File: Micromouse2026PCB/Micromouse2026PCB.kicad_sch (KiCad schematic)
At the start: 15 parts, among them J1 Power Terminal, J2 i2c OLED, J3 BNO085, SW1 RotaryEncoder_Switch, U6 L7805

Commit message: PCB work
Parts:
- J2: footprint Connector_PinHeader_2.54mm:PinHeader_1x04_P2.54mm_Vertical -> CustomFootprints:OLED_0.96_SSD1306_I2C
- J3: footprint Connector_PinHeader_2.54mm:PinHeader_1x06_P2.54mm_Vertical -> CustomFootprints:Adafruit_BNO085
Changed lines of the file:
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@@
 			)
 		)
-		(property "Footprint" "Connector_PinHeader_2.54mm:PinHeader_1x06_P2.54mm_Vertical"
+		(property "Footprint" "CustomFootprints:Adafruit_BNO085"
 			(at 101.6 48.26 0)
 			(hide yes)
@@
 			)
 		)
-		(property "Footprint" "Connector_PinHeader_2.54mm:PinHeader_1x04_P2.54mm_Vertical"
+		(property "Footprint" "CustomFootprints:OLED_0.96_SSD1306_I2C"
 			(at 101.6 69.85 0)
 			(hide yes)

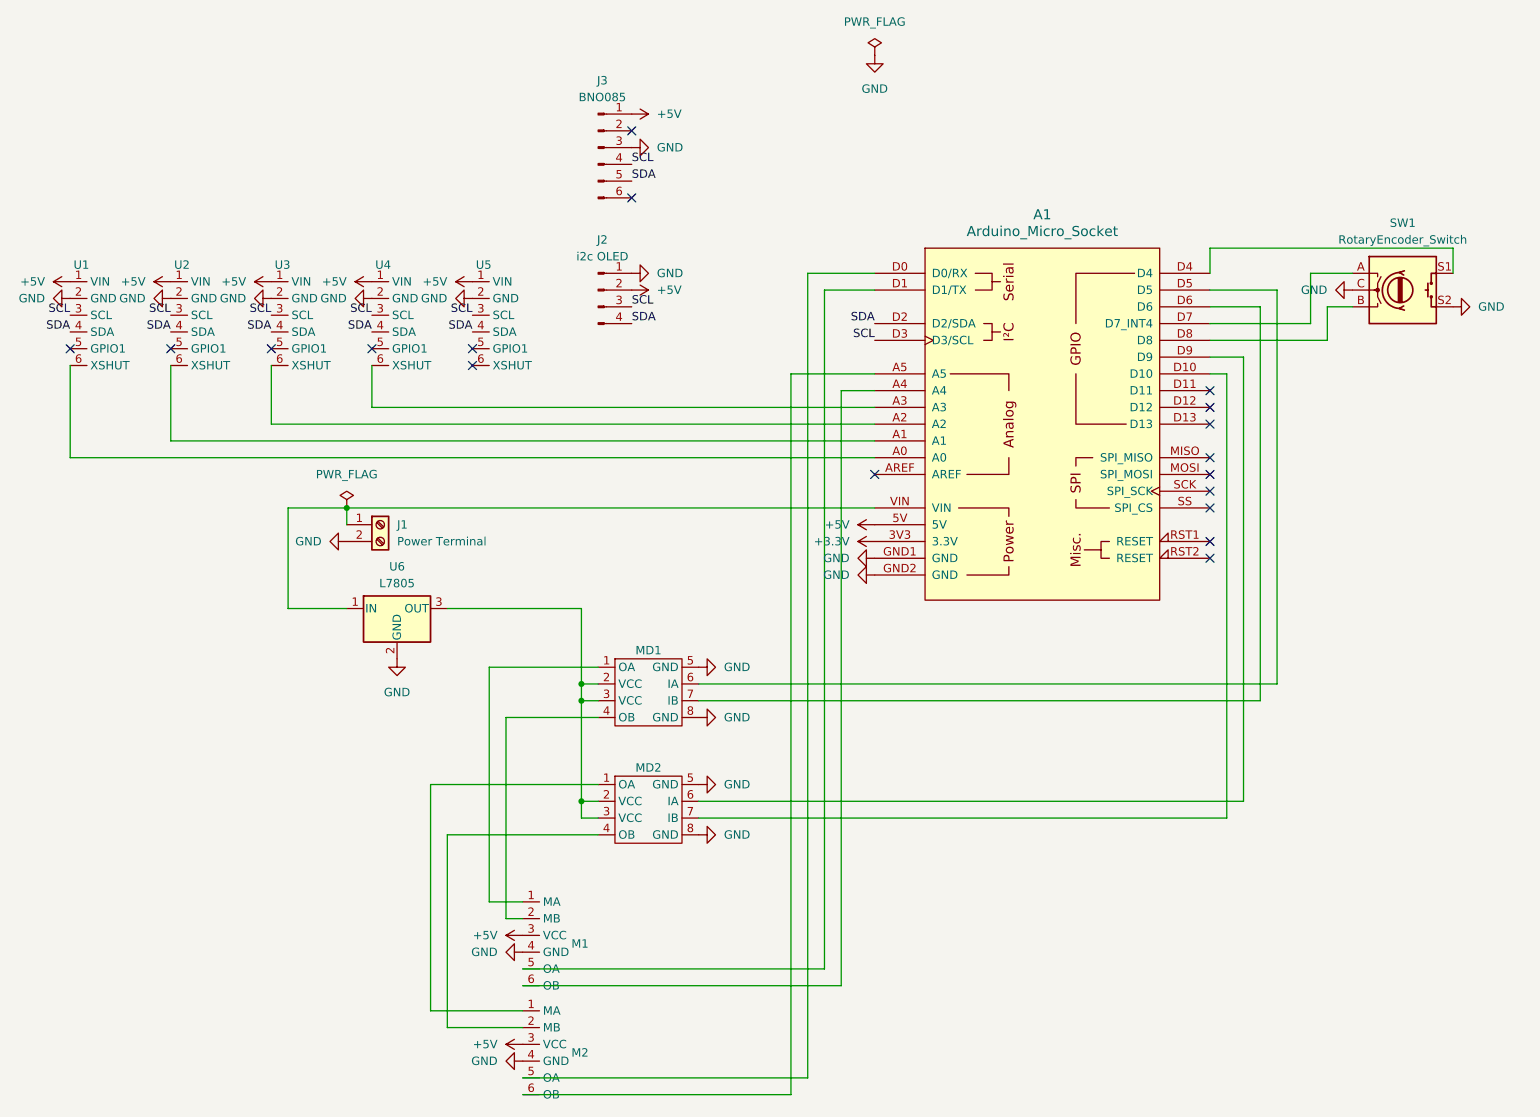
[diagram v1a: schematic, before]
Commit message: PCB working version
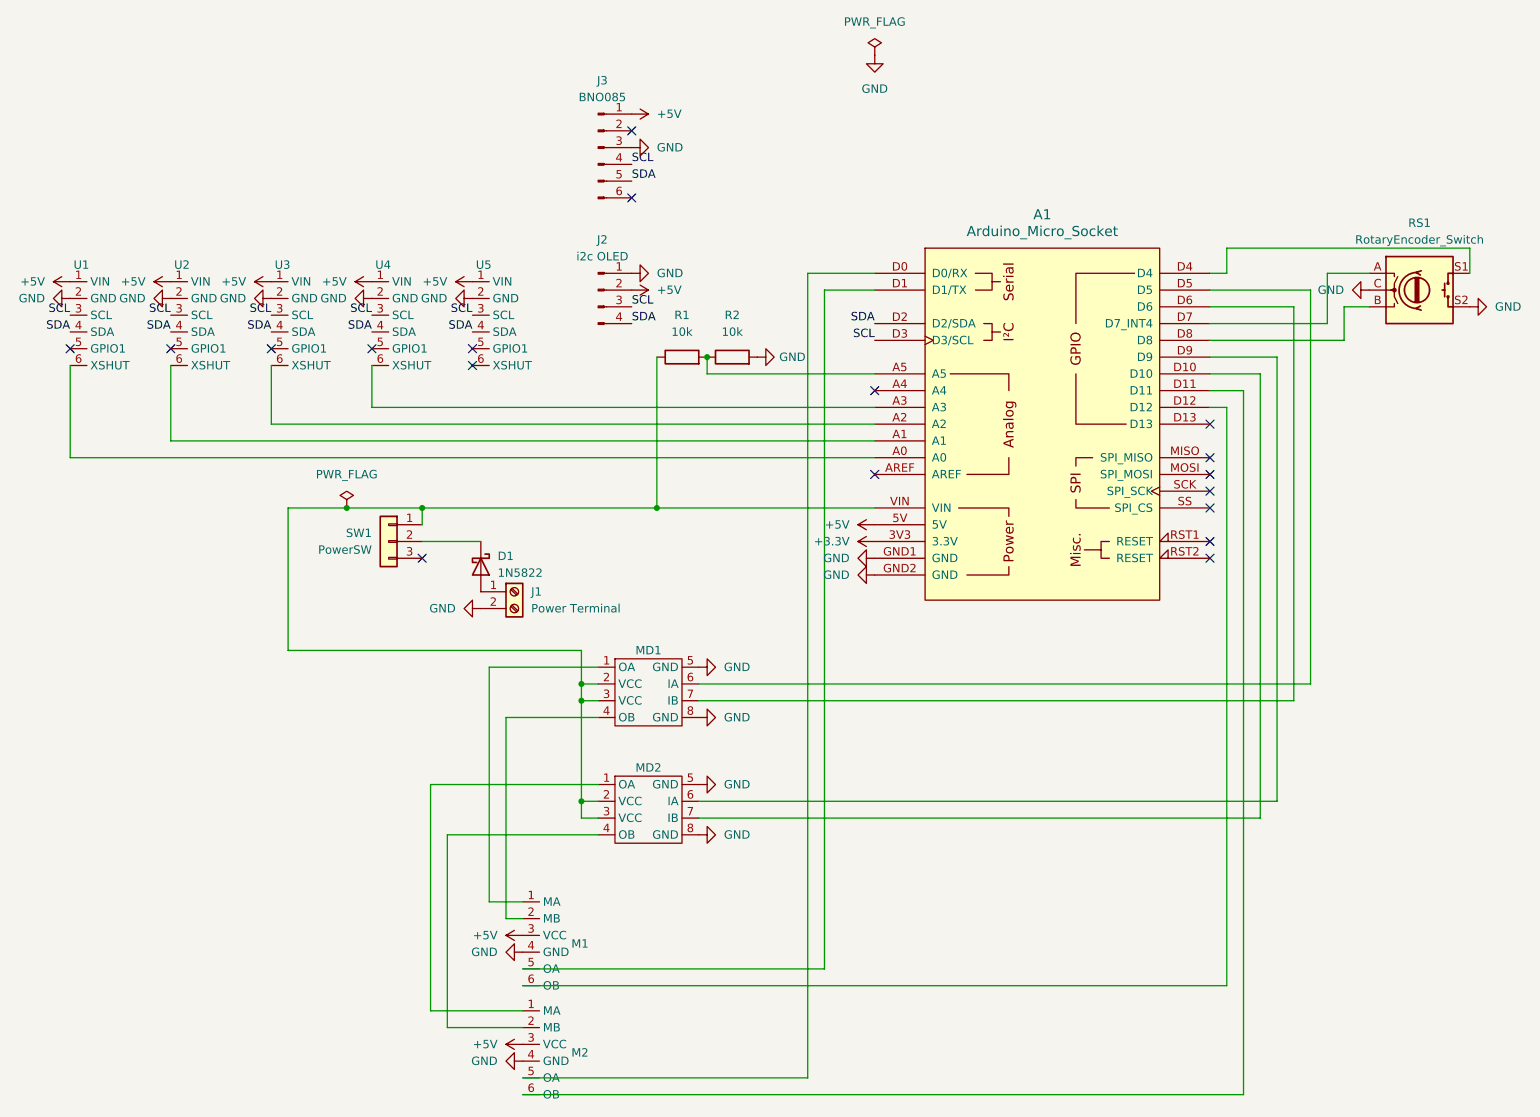
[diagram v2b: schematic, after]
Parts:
- removed U6: L7805, Package_TO_SOT_THT:TO-220-3_Vertical, symbol Regulator_Linear:L7805
- added D1: 1N5822, Diode_THT:D_DO-201AD_P15.24mm_Horizontal, symbol Diode:1N5822
- added R1, R2: 10k, Resistor_THT:R_Axial_DIN0207_L6.3mm_D2.5mm_P10.16mm_Horizontal, symbol Device:R
- added SW1: PowerSW, Connector_PinHeader_2.54mm:PinHeader_1x03_P2.54mm_Vertical, symbol Connector_Generic:Conn_01x03
- J1: footprint TerminalBlock_Phoenix:TerminalBlock_Phoenix_MKDS-1,5-2-5.08_1x02_P5.08mm_Horizontal -> TerminalBlock_Phoenix:TerminalBlock_Phoenix_MPT-0,5-2-2.54_1x02_P2.54mm_Horizontal
- renumbered SW1 to RS1
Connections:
- net GND: now also R2.2
- net at A1.A4: no longer M1.6 (OB)
- net at A1.A5: now also R1.2, R2.1; no longer M2.6 (OB)
- net at A1.D11: now also M2.6 (OB)
- net at A1.D12: now also M1.6 (OB)
- net at A1.VIN: now also MD1.2 (VCC), MD1.3 (VCC), MD2.2 (VCC), MD2.3 (VCC), R1.1, SW1.1 (Pin_1); no longer J1.1 (Pin_1)
- new net: D1.1 (K), SW1.2 (Pin_2)
- new net: D1.2 (A), J1.1 (Pin_1)
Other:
- moved on the sheet: J1, RS1
